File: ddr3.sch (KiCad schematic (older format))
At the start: 35 parts, among them U7 AS4C256M16D3, U8 TPS51200DRC

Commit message: Component placement done
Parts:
- R100, R99: renamed from R?; footprint antmicro-footprints:0402-res -> artix-dc-scm-footprints:0402-res; symbol antmicroResistors0402:R_51R_0402 -> artix-dc-scm:R_51R_0402
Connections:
- net DDR3_CLK+: now also R99.2; no longer R99.1
- net at C63.2, R100.1: now also R99.1; no longer R99.2
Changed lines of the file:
@@
 DDR3_VTT
 $Comp
-L antmicroResistors0402:R_51R_0402 R?
+L artix-dc-scm:R_51R_0402 R99
 U 1 1 5FDBE47E
 P 12475 8050
-F 0 "R?" V 12430 8120 60  0000 L CNN
+F 0 "R99" V 12430 8120 60  0000 L CNN
 F 1 "R_51R_0402" H 12475 7900 60  0001 C CNN
-F 2 "antmicro-footprints:0402-res" H 12675 8250 60  0001 L CNN
+F 2 "artix-dc-scm-footprints:0402-res" H 12675 8250 60  0001 L CNN
 F 3 "" H 12475 8050 50  0001 C CNN
 F 4 "YAGEO" H 12675 8450 60  0001 L CNN "Manufacturer"
@@
 F 6 "51R" V 12528 8120 50  0000 L CNN "Val"
 	1    12475 8050
-	0    1    1    0
+	0    1    -1   0
 $EndComp
 $Comp
-L antmicroResistors0402:R_51R_0402 R?
+L artix-dc-scm:R_51R_0402 R100
 U 1 1 5FDBF551
 P 12475 8450
-F 0 "R?" V 12430 8520 60  0000 L CNN
+F 0 "R100" V 12430 8520 60  0000 L CNN
 F 1 "R_51R_0402" H 12475 8300 60  0001 C CNN
-F 2 "antmicro-footprints:0402-res" H 12675 8650 60  0001 L CNN
+F 2 "artix-dc-scm-footprints:0402-res" H 12675 8650 60  0001 L CNN
 F 3 "" H 12475 8450 50  0001 C CNN
 F 4 "YAGEO" H 12675 8850 60  0001 L CNN "Manufacturer"

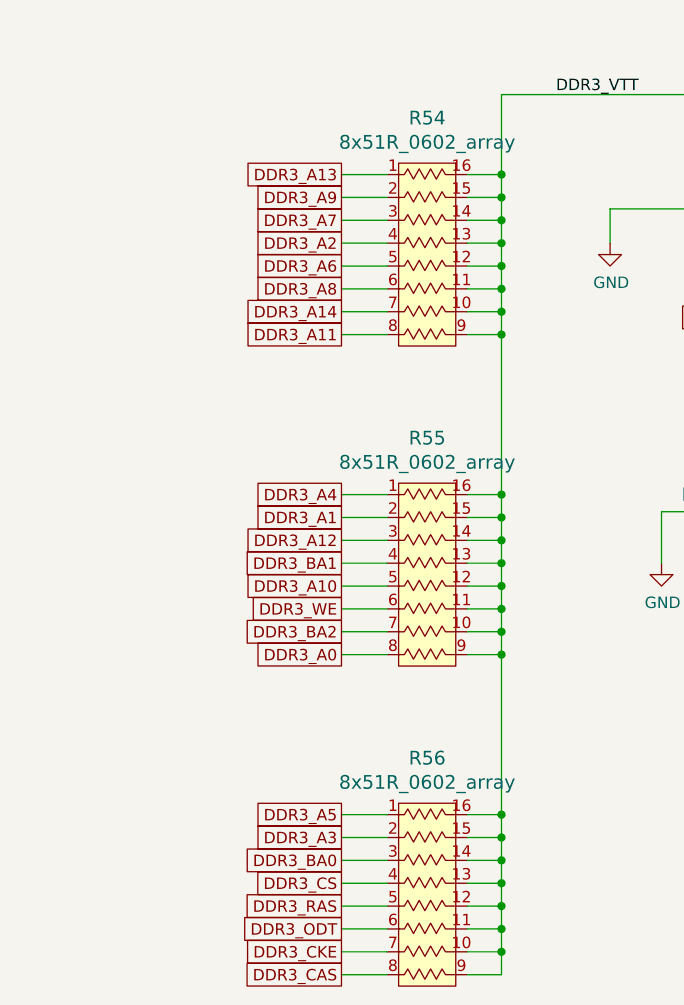
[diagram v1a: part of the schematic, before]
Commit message: Improved DDR3 related connection (WIP)
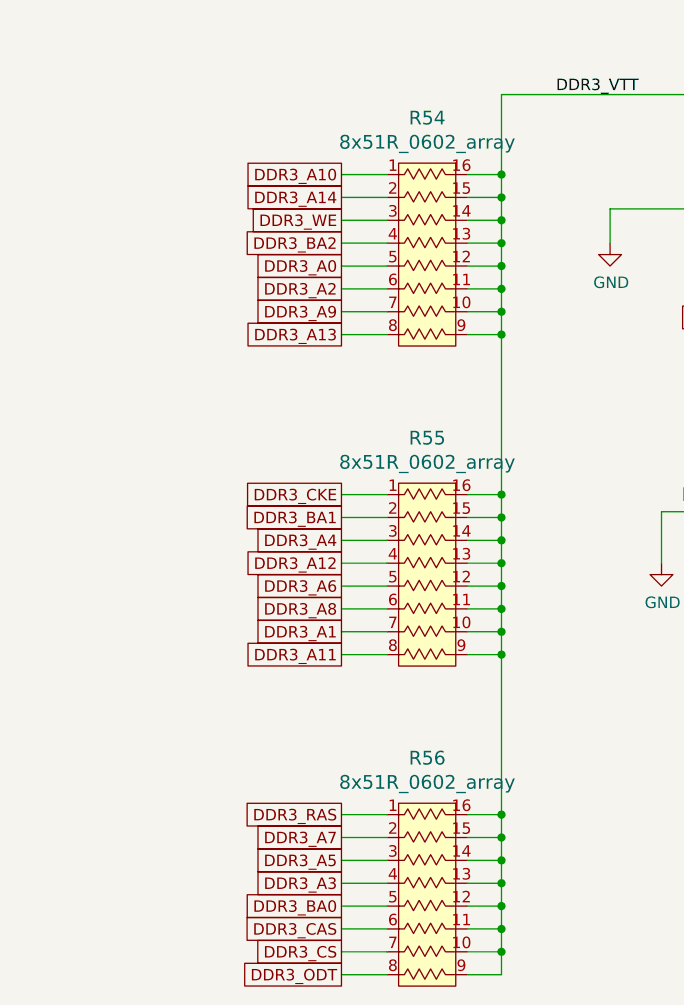
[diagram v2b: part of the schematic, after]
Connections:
- net DDR3_A0: now also R54.5; no longer R55.8
- net DDR3_A1: now also R55.7; no longer R55.2
- net DDR3_A10: now also R54.1; no longer R55.5
- net DDR3_A11: now also R55.8; no longer R54.8
- net DDR3_A12: now also R55.4; no longer R55.3
- net DDR3_A13: now also R54.8; no longer R54.1
- net DDR3_A14: now also R54.2; no longer R54.7
- net DDR3_A2: now also R54.6; no longer R54.4
- net DDR3_A3: now also R56.4; no longer R56.2
- net DDR3_A4: now also R55.3; no longer R55.1
- net DDR3_A5: now also R56.3; no longer R56.1
- net DDR3_A6: now also R55.5; no longer R54.5
- net DDR3_A7: now also R56.2; no longer R54.3
- net DDR3_A8: now also R55.6; no longer R54.6
- net DDR3_A9: now also R54.7; no longer R54.2
- net DDR3_BA0: now also R56.5; no longer R56.3
- net DDR3_BA1: now also R55.2; no longer R55.4
- net DDR3_BA2: now also R54.4; no longer R55.7
- net DDR3_CAS: now also R56.6; no longer R56.8
- net DDR3_CKE: now also R55.1; no longer R56.7
- net DDR3_CS: now also R56.7; no longer R56.4
- net DDR3_ODT: now also R56.8; no longer R56.6
- net DDR3_RAS: now also R56.1; no longer R56.5
- net DDR3_WE: now also R54.3; no longer R55.6
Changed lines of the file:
@@
 Wire Wire Line
 	11775 2375 11775 2700
+Text GLabel 4425 9375 0    50   UnSpc ~ 0
+DDR3_A1
+Text GLabel 4425 8975 0    50   UnSpc ~ 0
+DDR3_A4
+Text GLabel 4425 9175 0    50   UnSpc ~ 0
+DDR3_A6
+Text GLabel 4425 9275 0    50   UnSpc ~ 0
+DDR3_A8
 Text GLabel 4425 9475 0    50   UnSpc ~ 0
-DDR3_A0
+DDR3_A11
+Text GLabel 4425 9075 0    50   UnSpc ~ 0
+DDR3_A12
+Text GLabel 4425 7475 0    50   UnSpc ~ 0
+DDR3_A14
+Wire Wire Line
+	4425 9475 4625 9475
+Wire Wire Line
+	4625 8875 4425 8875
+Wire Wire Line
+	4625 7675 4425 7675
+Wire Wire Line
+	4625 10275 4425 10275
+Wire Wire Line
+	4425 8775 4625 8775
+Wire Wire Line
+	4425 10175 4625 10175
+Wire Wire Line
+	4425 7775 4625 7775
+Wire Wire Line
+	4425 7575 4625 7575
+Wire Wire Line
+	4425 7875 4625 7875
+Wire Wire Line
+	4425 7475 4625 7475
+Wire Wire Line
+	4425 9175 4625 9175
+Wire Wire Line
+	4425 8075 4625 8075
+Wire Wire Line
+	4425 8975 4625 8975
+Wire Wire Line
+	4425 7375 4625 7375
+Wire Wire Line
+	4425 7975 4625 7975
 Text GLabel 4425 8875 0    50   UnSpc ~ 0
-DDR3_A1
-Text GLabel 4425 7675 0    50   UnSpc ~ 0
-DDR3_A2
-Text GLabel 4425 10275 0    50   UnSpc ~ 0
-DDR3_A3
-Text GLabel 4425 8775 0    50   UnSpc ~ 0
-DDR3_A4
-Text GLabel 4425 10175 0    50   UnSpc ~ 0
-DDR3_A5
-Text GLabel 4425 7775 0    50   UnSpc ~ 0
-DDR3_A6
-Text GLabel 4425 7575 0    50   UnSpc ~ 0
-DDR3_A7
-Text GLabel 4425 7875 0    50   UnSpc ~ 0
-DDR3_A8
-Text GLabel 4425 7475 0    50   UnSpc ~ 0
-DDR3_A9
-Text GLabel 4425 9175 0    50   UnSpc ~ 0
-DDR3_A10
-Text GLabel 4425 8075 0    50   UnSpc ~ 0
-DDR3_A11
-Text GLabel 4425 8975 0    50   UnSpc ~ 0
-DDR3_A12
-Text GLabel 4425 7375 0    50   UnSpc ~ 0
-DDR3_A13
-Text GLabel 4425 7975 0    50   UnSpc ~ 0
-DDR3_A14
-Wire Wire Line
-	4425 9475 4625 9475
-Wire Wire Line
-	4625 8875 4425 8875
-Wire Wire Line
-	4625 7675 4425 7675
-Wire Wire Line
-	4625 10275 4425 10275
-Wire Wire Line
-	4425 8775 4625 8775
-Wire Wire Line
-	4425 10175 4625 10175
-Wire Wire Line
-	4425 7775 4625 7775
-Wire Wire Line
-	4425 7575 4625 7575
-Wire Wire Line
-	4425 7875 4625 7875
-Wire Wire Line
-	4425 7475 4625 7475
-Wire Wire Line
-	4425 9175 4625 9175
-Wire Wire Line
-	4425 8075 4625 8075
-Wire Wire Line
-	4425 8975 4625 8975
-Wire Wire Line
-	4425 7375 4625 7375
-Wire Wire Line
-	4425 7975 4625 7975
-Text GLabel 4425 10375 0    50   UnSpc ~ 0
-DDR3_BA0
-Text GLabel 4425 9075 0    50   UnSpc ~ 0
 DDR3_BA1
-Text GLabel 4425 9375 0    50   UnSpc ~ 0
-DDR3_BA2
 Wire Wire Line
 	4425 10375 4625 10375
@@
 Wire Wire Line
 	4425 9375 4625 9375
-Text GLabel 4425 10575 0    50   UnSpc ~ 0
-DDR3_RAS
-Text GLabel 4425 10875 0    50   UnSpc ~ 0
-DDR3_CAS
 Wire Wire Line
 	4425 10875 4625 10875
 Wire Wire Line
 	4625 10575 4425 10575
-Text GLabel 4425 9275 0    50   UnSpc ~ 0
-DDR3_WE
-Text GLabel 4425 10475 0    50   UnSpc ~ 0
-DDR3_CS
 Wire Wire Line
 	4625 9275 4425 9275
 Wire Wire Line
 	4425 10475 4625 10475
-Text GLabel 4425 10775 0    50   UnSpc ~ 0
-DDR3_CKE
-Text GLabel 4425 10675 0    50   UnSpc ~ 0
-DDR3_ODT
 Wire Wire Line
 	4425 10675 4625 10675
@@
 	0    1    1    0
 $EndComp
+Text GLabel 4425 10875 0    50   UnSpc ~ 0
+DDR3_ODT
+Text GLabel 4425 8775 0    50   UnSpc ~ 0
+DDR3_CKE
+Text GLabel 4425 10775 0    50   UnSpc ~ 0
+DDR3_CS
+Text GLabel 4425 10675 0    50   UnSpc ~ 0
+DDR3_CAS
+Text GLabel 4425 10175 0    50   UnSpc ~ 0
+DDR3_RAS
+Text GLabel 4425 10575 0    50   UnSpc ~ 0
+DDR3_BA0
+Text GLabel 4425 10475 0    50   UnSpc ~ 0
+DDR3_A3
+Text GLabel 4425 7575 0    50   UnSpc ~ 0
+DDR3_WE
+Text GLabel 4425 7675 0    50   UnSpc ~ 0
+DDR3_BA2
+Text GLabel 4425 10275 0    50   UnSpc ~ 0
+DDR3_A7
+Text GLabel 4425 7875 0    50   UnSpc ~ 0
+DDR3_A2
+Text GLabel 4425 7775 0    50   UnSpc ~ 0
+DDR3_A0
+Text GLabel 4425 10375 0    50   UnSpc ~ 0
+DDR3_A5
+Text GLabel 4425 7375 0    50   UnSpc ~ 0
+DDR3_A10
+Text GLabel 4425 8075 0    50   UnSpc ~ 0
+DDR3_A13
+Text GLabel 4425 7975 0    50   UnSpc ~ 0
+DDR3_A9
 $EndSCHEMATC
